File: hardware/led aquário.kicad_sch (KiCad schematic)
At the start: 50 parts, among them J1 Conn_01x01, J2 Conn_01x01, J3 Conn_01x01, J4 Conn_01x01, J5 Conn_01x01, J6 Conn_01x01, J7 Conn_01x01, J8 Conn_01x01

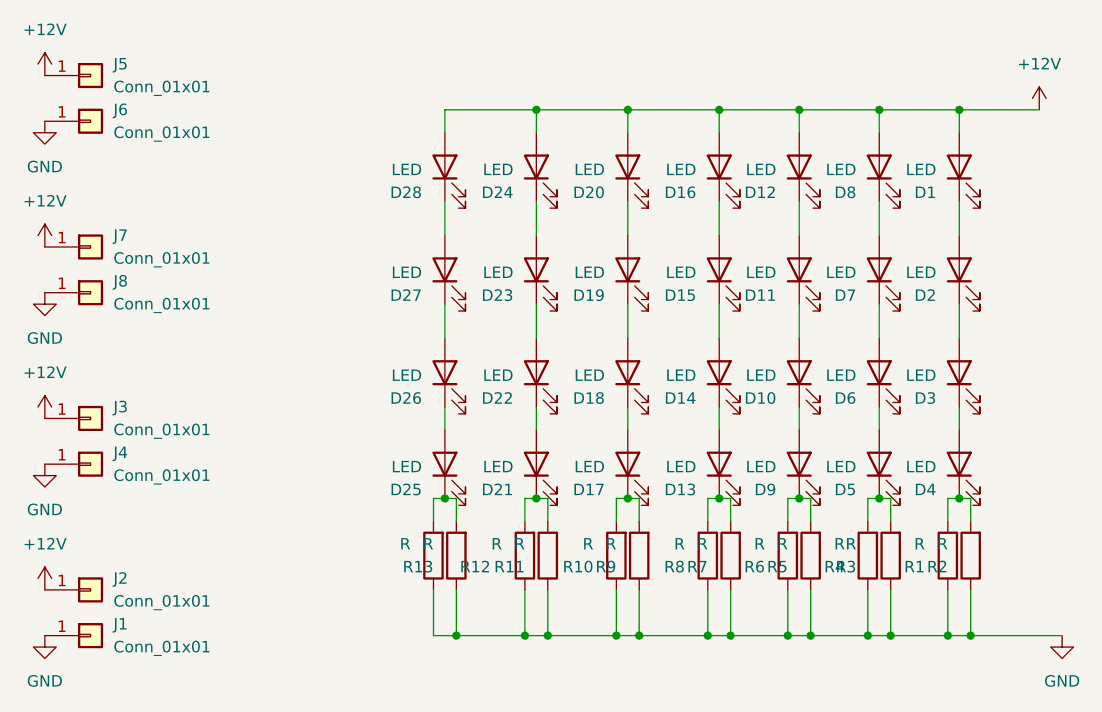
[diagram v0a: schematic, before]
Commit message: att
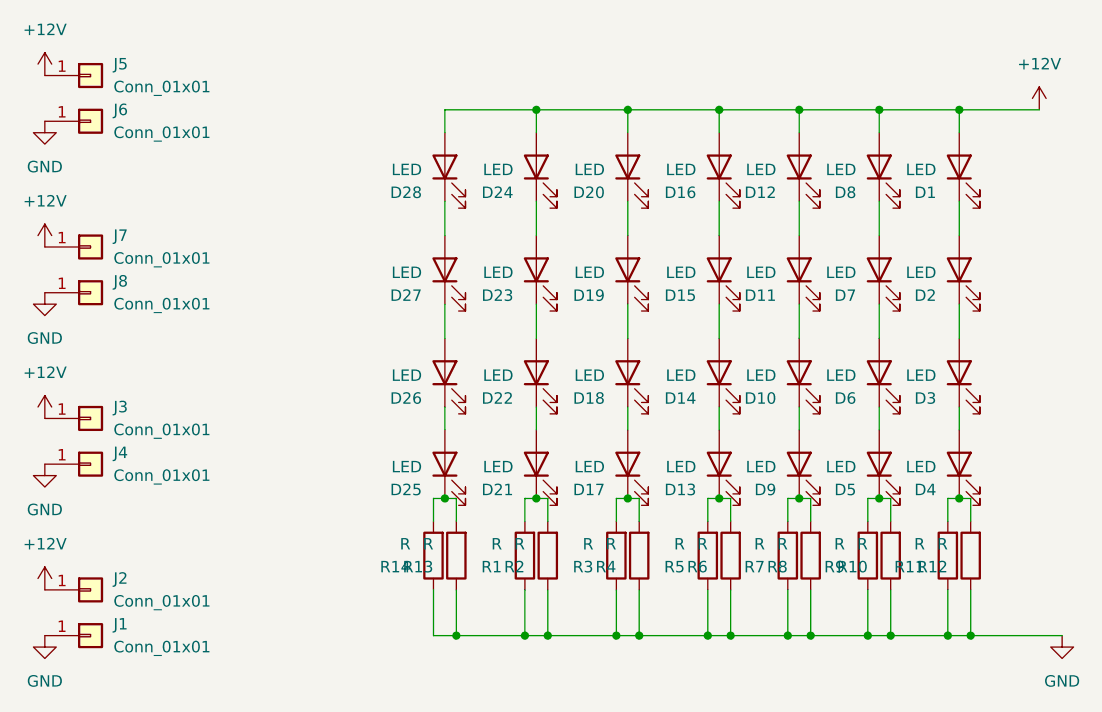
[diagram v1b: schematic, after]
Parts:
- J1, J2, J3, J4, J5, J6, J7, J8: footprint TestPoint:TestPoint_THTPad_4.0x4.0mm_Drill2.0mm -> TestPoint:TestPoint_Pad_4.0x4.0mm
- R1, R10, R11, R12, R13, R14, R2, R3, R4, R5, R6, R7, R8, R9: footprint Resistor_SMD:R_1206_3216Metric -> Resistor_SMD:R_2512_6332Metric
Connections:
- net at R7.2, R8.2: now also D9.1 (K); no longer D13.1 (K)
- net at R11.2, R12.2: now also D4.1 (K); no longer D21.1 (K)
- net at R3.2, R4.2: now also D17.1 (K); no longer D5.1 (K)
- net at R1.2, R2.2: now also D21.1 (K); no longer D4.1 (K)
- net at R5.2, R6.2: now also D13.1 (K); no longer D9.1 (K)
- net at R10.2, R9.2: now also D5.1 (K); no longer D17.1 (K)
